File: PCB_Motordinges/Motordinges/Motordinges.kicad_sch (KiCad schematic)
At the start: 22 parts, among them J1 Conn_01x04_Pin, J2 Barrel_Jack, SW1 EN, SW2 FLASH, U1 ESP32-WROOM-32, U2 MP1584, U3 AMS1117-3.3

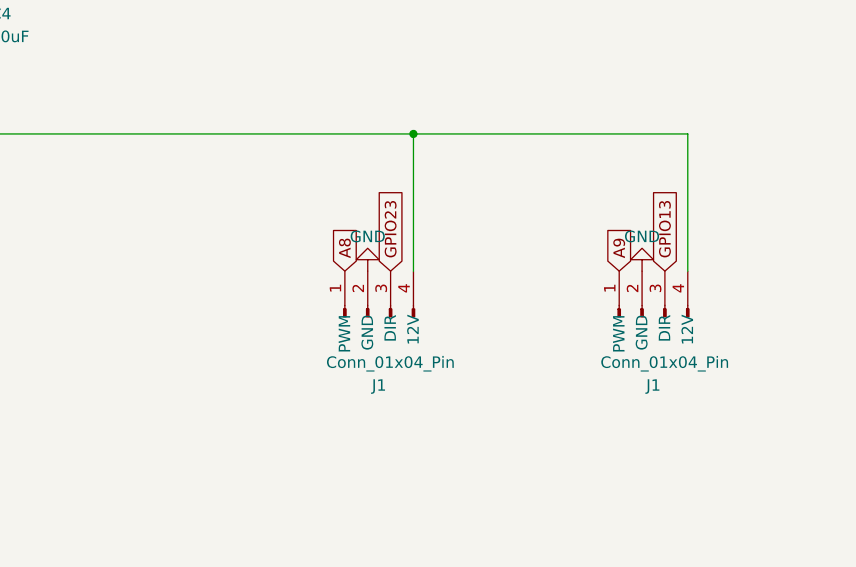
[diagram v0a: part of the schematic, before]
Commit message: pcb_v2
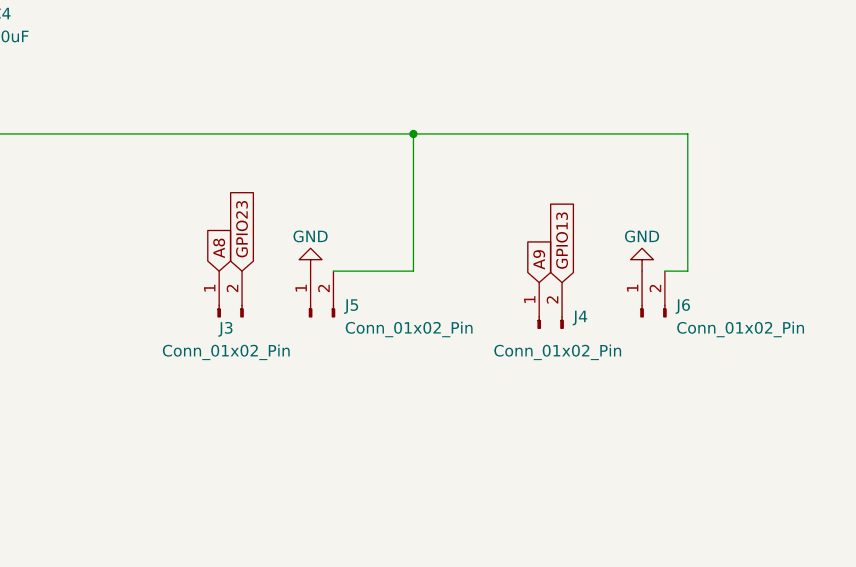
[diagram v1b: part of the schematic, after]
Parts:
- removed J1 (x2): Conn_01x04_Pin, Connector_PinHeader_2.00mm:PinHeader_1x04_P2.00mm_Vertical, symbol Connector:Conn_01x04_Pin
- added J3, J4: Conn_01x02_Pin, Connector_PinHeader_2.54mm:PinHeader_1x02_P2.54mm_Vertical, symbol Connector:Conn_01x02_Pin
- added J5, J6: Conn_01x02_Pin, TerminalBlock:TerminalBlock_bornier-2_P5.08mm, symbol Connector:Conn_01x02_Pin
- J1: footprint Connector_PinHeader_2.00mm:PinHeader_1x04_P2.00mm_Vertical -> Connector_PinHeader_2.54mm:PinHeader_1x04_P2.54mm_Vertical
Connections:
- net A8: now also J3.1 (Pin_1)
- net A9: now also J4.1 (Pin_1)
- net GND: now also J5.1 (Pin_1), J6.1 (Pin_1)
- net GPIO13: now also J4.2 (Pin_2)
- net GPIO23: now also J3.2 (Pin_2)
- net at J2.1, U2.3 (IN+), U2.4 (IN+): now also J5.2 (Pin_2), J6.2 (Pin_2)
